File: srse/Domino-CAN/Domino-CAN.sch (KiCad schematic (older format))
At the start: 1 part, among them U1 DOMINO_DOMINO

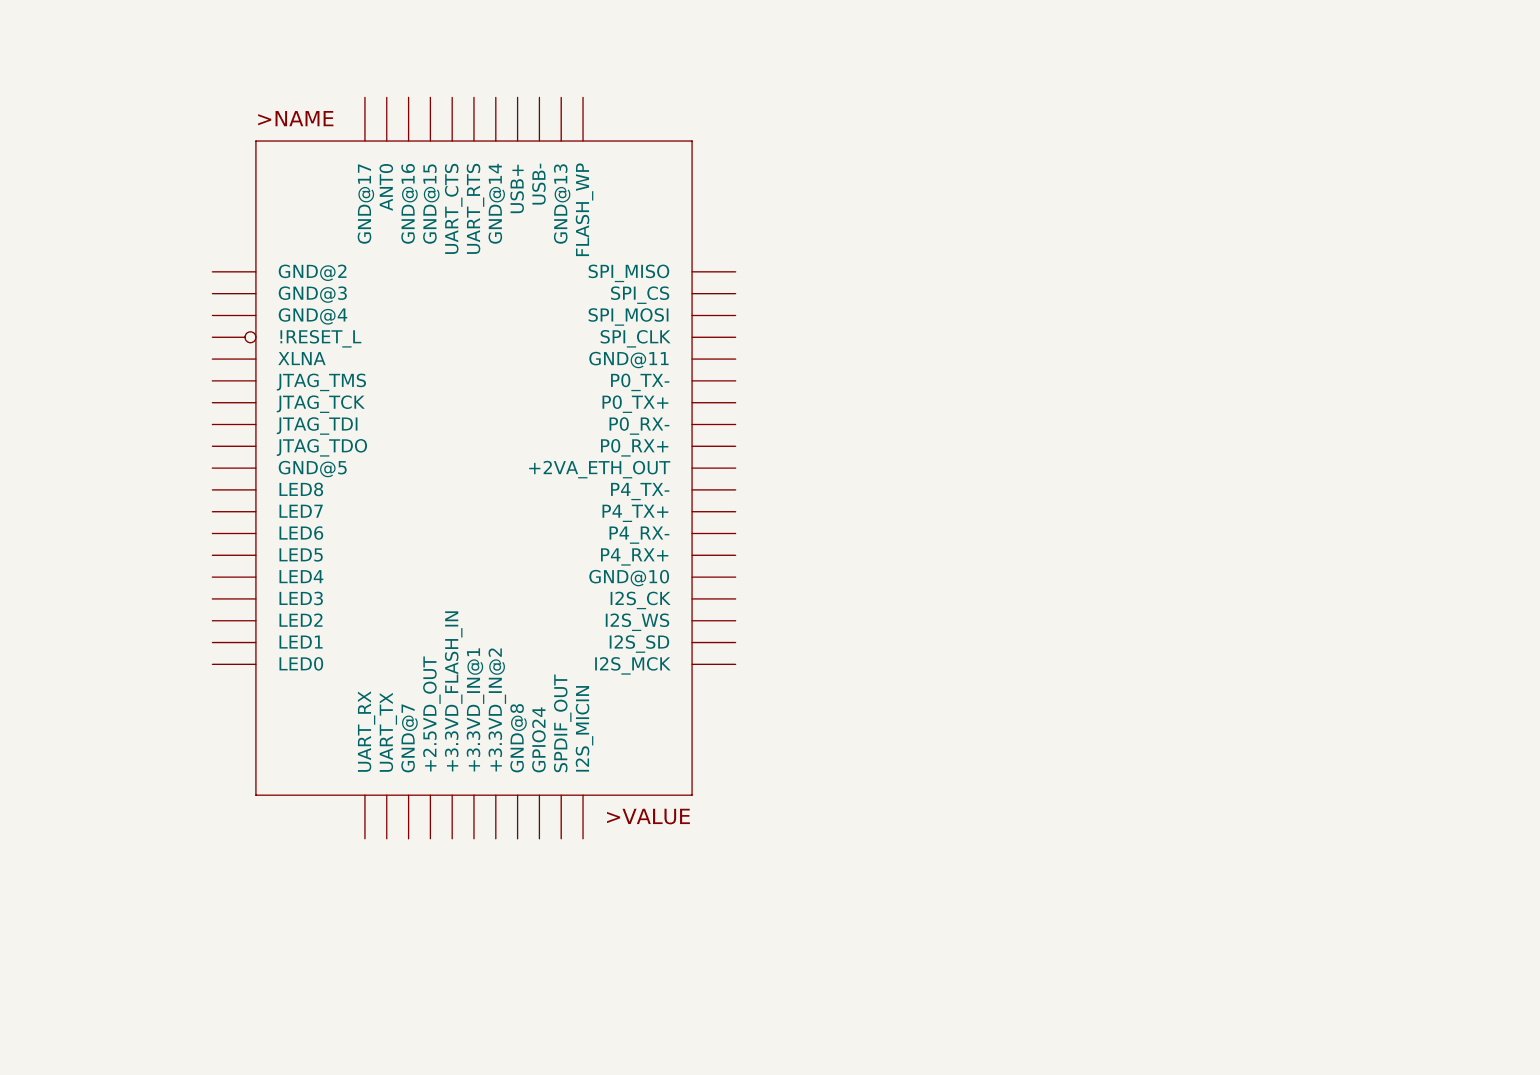
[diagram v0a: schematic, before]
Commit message: Domino-CAN wip
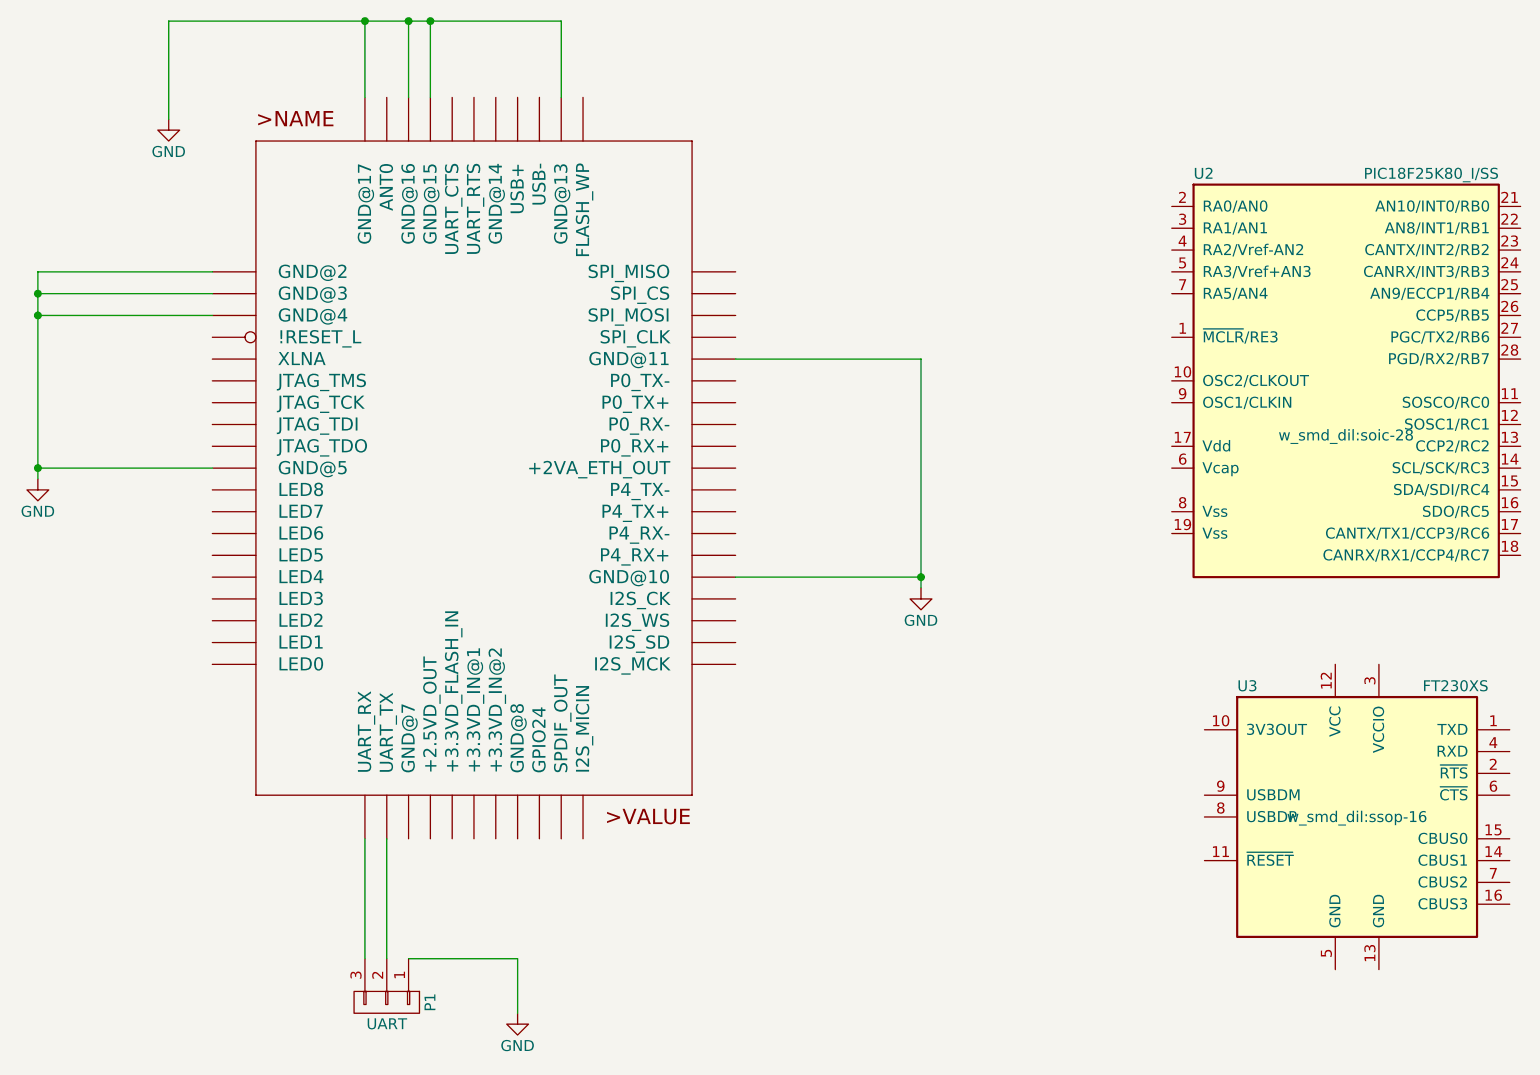
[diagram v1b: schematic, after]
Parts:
- added P1: UART, Pin_Headers:Pin_Header_Straight_1x03, symbol CONN_01X03
- added U2: PIC18F25K80_I/SS, w_smd_dil:soic-28, symbol PIC18F25K80_I/SS
- added U3: FT230XS, w_smd_dil:ssop-16, symbol FT230XS
- U1: value DOMINO_DOMINO -> DOMINO_CORE
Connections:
- net GND: now reaches U1.1 (GND@2)
- net GND: now also U1.10 (GND@5), U1.2 (GND@3), U1.3 (GND@4), U1.35 (GND@10), U1.45 (GND@11), U1.51 (GND@13), U1.57 (GND@15), U1.58 (GND@16), U1.60 (GND@17), P1.1 (P1)
- net at U1.20 (UART_RX): now also P1.3 (P3)
- net at U1.21 (UART_TX): now also P1.2 (P2)
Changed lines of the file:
@@
 LIBS:contrib
 LIBS:valves
-LIBS:Domino
+LIBS:microchip_pic18mcu
+LIBS:ftdi
 LIBS:Domino-CAN-cache
 EELAYER 25 0
@@
 P 6300 3600
 F 0 "U1" H 6300 3600 60  0001 C CNN
-F 1 "DOMINO_DOMINO" H 6300 3600 60  0001 C CNN
+F 1 "DOMINO_CORE" H 6300 3600 60  0001 C CNN
 F 2 "Domino:DOMINO" H 6300 3600 60  0001 C CNN
 F 3 "" H 6300 3600 60  0000 C CNN
@@
 	1    0    0    -1
 $EndComp
+$Comp
+L CONN_01X03 P1
+U 1 1 56AE17B3
+P 4500 6150
+F 0 "P1" H 4500 6350 50  0000 C CNN
+F 1 "UART" V 4600 6150 50  0000 C CNN
+F 2 "Pin_Headers:Pin_Header_Straight_1x03" H 4500 6150 50  0001 C CNN
+F 3 "" H 4500 6150 50  0000 C CNN
+	1    4500 6150
+	0    1    1    0
+$EndComp
+$Comp
+L GND #PWR01
+U 1 1 56AE1870
+P 5100 6200
+F 0 "#PWR01" H 5100 5950 50  0001 C CNN
+F 1 "GND" H 5100 6050 50  0000 C CNN
+F 2 "" H 5100 6200 50  0000 C CNN
+F 3 "" H 5100 6200 50  0000 C CNN
+	1    5100 6200
+	1    0    0    -1
+$EndComp
+$Comp
+L GND #PWR02
+U 1 1 56AE1A1C
+P 2900 3750
+F 0 "#PWR02" H 2900 3500 50  0001 C CNN
+F 1 "GND" H 2900 3600 50  0000 C CNN
+F 2 "" H 2900 3750 50  0000 C CNN
+F 3 "" H 2900 3750 50  0000 C CNN
+	1    2900 3750
+	1    0    0    -1
+$EndComp
+Wire Wire Line
+	4400 5400 4400 5950
+Wire Wire Line
+	4500 5400 4500 5950
+Wire Wire Line
+	4600 5950 5100 5950
+Wire Wire Line
+	5100 5950 5100 6200
+Wire Wire Line
+	2900 3000 3700 3000
+Wire Wire Line
+	2900 2800 2900 3750
+Wire Wire Line
+	3700 2900 2900 2900
+Connection ~ 2900 3000
+Wire Wire Line
+	3700 2800 2900 2800
+Connection ~ 2900 2900
+$Comp
+L GND #PWR03
+U 1 1 56AE1ABA
+P 3500 2100
+F 0 "#PWR03" H 3500 1850 50  0001 C CNN
+F 1 "GND" H 3500 1950 50  0000 C CNN
+F 2 "" H 3500 2100 50  0000 C CNN
+F 3 "" H 3500 2100 50  0000 C CNN
+	1    3500 2100
+	1    0    0    -1
+$EndComp
+Wire Wire Line
+	4400 2000 4400 1650
+Wire Wire Line
+	3500 1650 5300 1650
+Wire Wire Line
+	3500 1650 3500 2100
+Wire Wire Line
+	4600 1650 4600 2000
+Connection ~ 4400 1650
+Wire Wire Line
+	4700 1650 4700 2000
+Connection ~ 4600 1650
+Wire Wire Line
+	5300 1650 5300 2000
+Connection ~ 4700 1650
+$Comp
+L GND #PWR04
+U 1 1 56AE1B90
+P 6950 4250
+F 0 "#PWR04" H 6950 4000 50  0001 C CNN
+F 1 "GND" H 6950 4100 50  0000 C CNN
+F 2 "" H 6950 4250 50  0000 C CNN
+F 3 "" H 6950 4250 50  0000 C CNN
+	1    6950 4250
+	1    0    0    -1
+$EndComp
+Wire Wire Line
+	6100 4200 6950 4200
+Wire Wire Line
+	6950 3200 6950 4250
+Wire Wire Line
+	6100 3200 6950 3200
+Connection ~ 6950 4200
+Wire Wire Line
+	2900 3700 3700 3700
+Connection ~ 2900 3700
+$Comp
+L PIC18F25K80_I/SS U2
+U 1 1 56AE1E68
+P 8900 3300
+F 0 "U2" H 8200 4250 50  0000 L CNN
+F 1 "PIC18F25K80_I/SS" H 9600 4250 50  0000 R CNN
+F 2 "w_smd_dil:soic-28" H 8900 3050 50  0000 C CNN
+F 3 "" H 8900 3250 50  0000 C CNN
+	1    8900 3300
+	1    0    0    -1
+$EndComp
+$Comp
+L FT230XS U3
+U 1 1 56AE1F4F
+P 8950 5300
+F 0 "U3" H 8400 5900 50  0000 L CNN
+F 1 "FT230XS" H 9250 5900 50  0000 L CNN
+F 2 "w_smd_dil:ssop-16" H 8950 5300 50  0000 C CNN
+F 3 "" H 8950 5300 50  0000 C CNN
+	1    8950 5300
+	1    0    0    -1
+$EndComp
